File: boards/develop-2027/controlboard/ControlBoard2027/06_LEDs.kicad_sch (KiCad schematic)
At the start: 12 parts, among them U7 74AHCT125

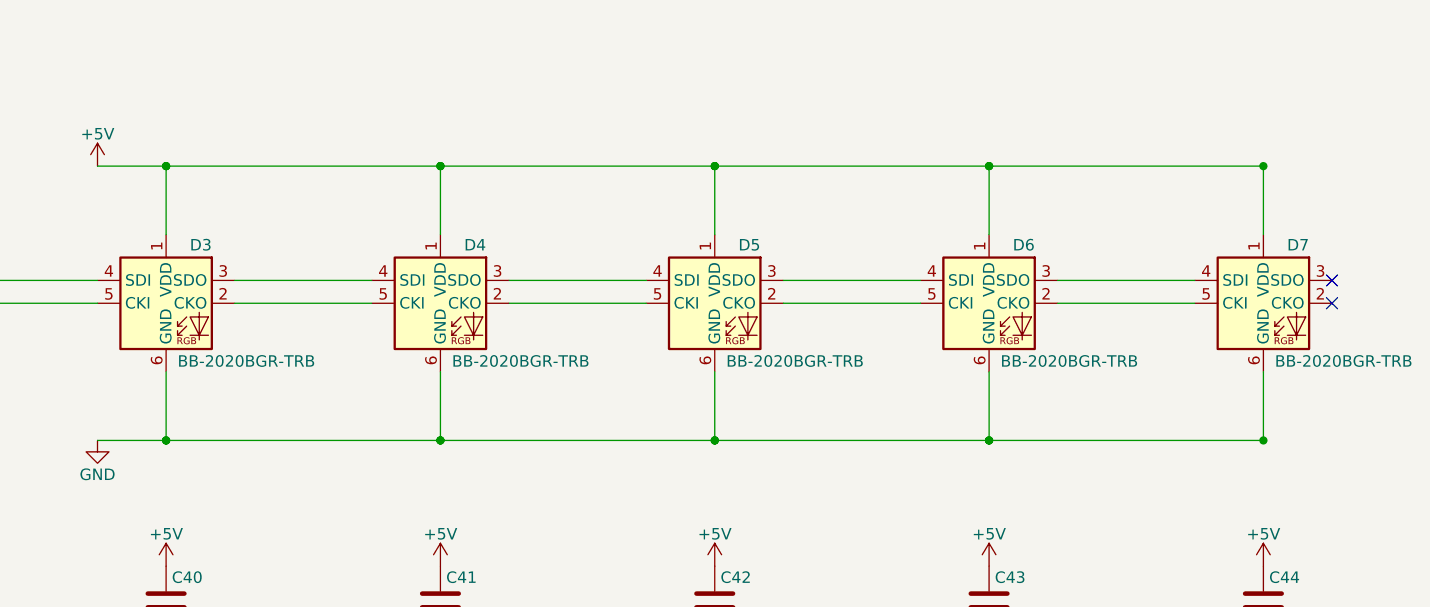
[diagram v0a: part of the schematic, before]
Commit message: features....
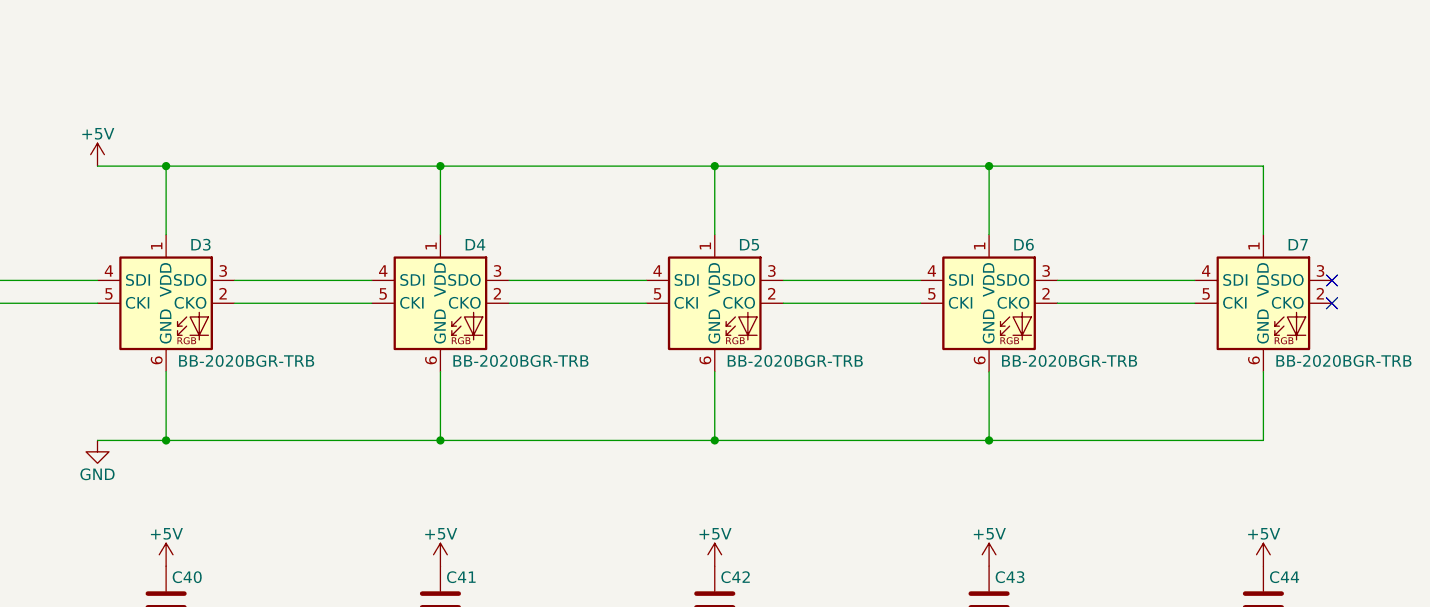
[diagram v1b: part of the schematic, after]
